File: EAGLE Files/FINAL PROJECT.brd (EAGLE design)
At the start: 100.3 x 49.5 mm, 15 parts, among them J1 BATTERY, U1 9_to_3.3_VREG

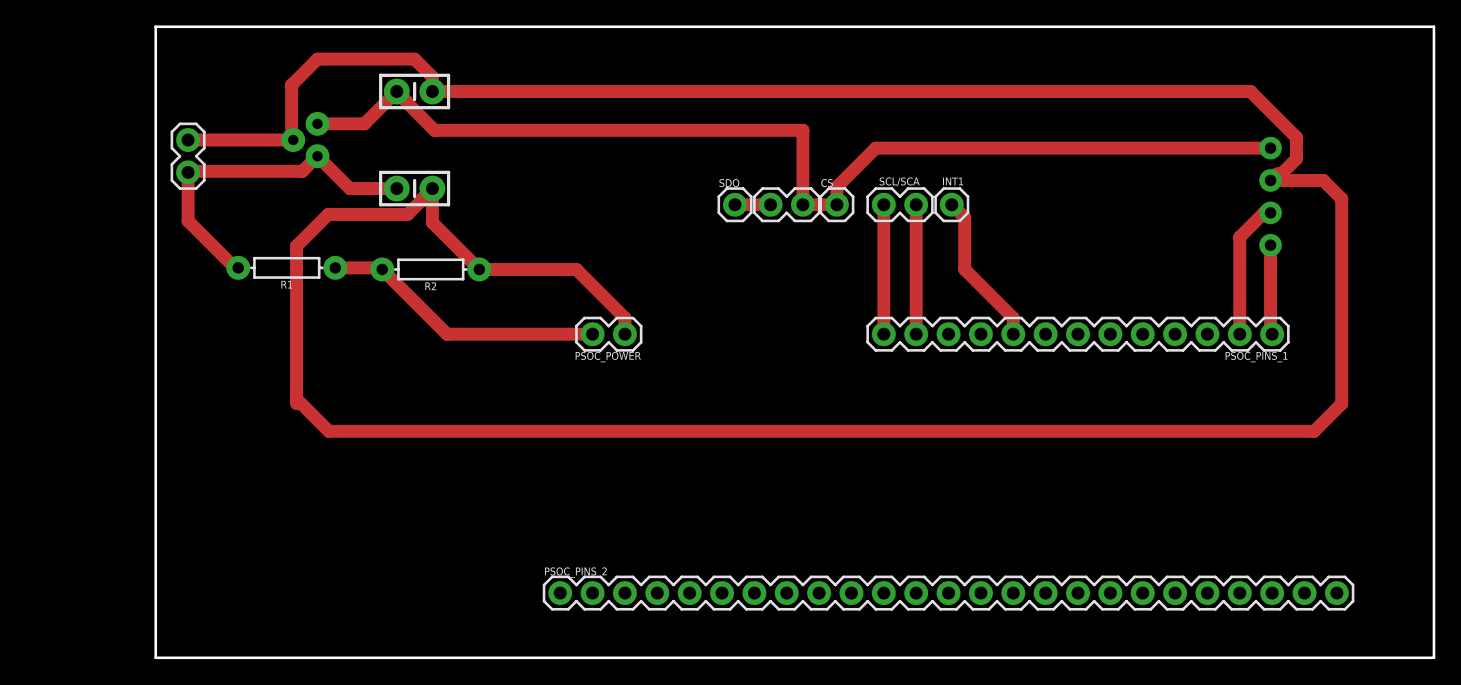
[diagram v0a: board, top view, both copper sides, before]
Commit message: FS and So code
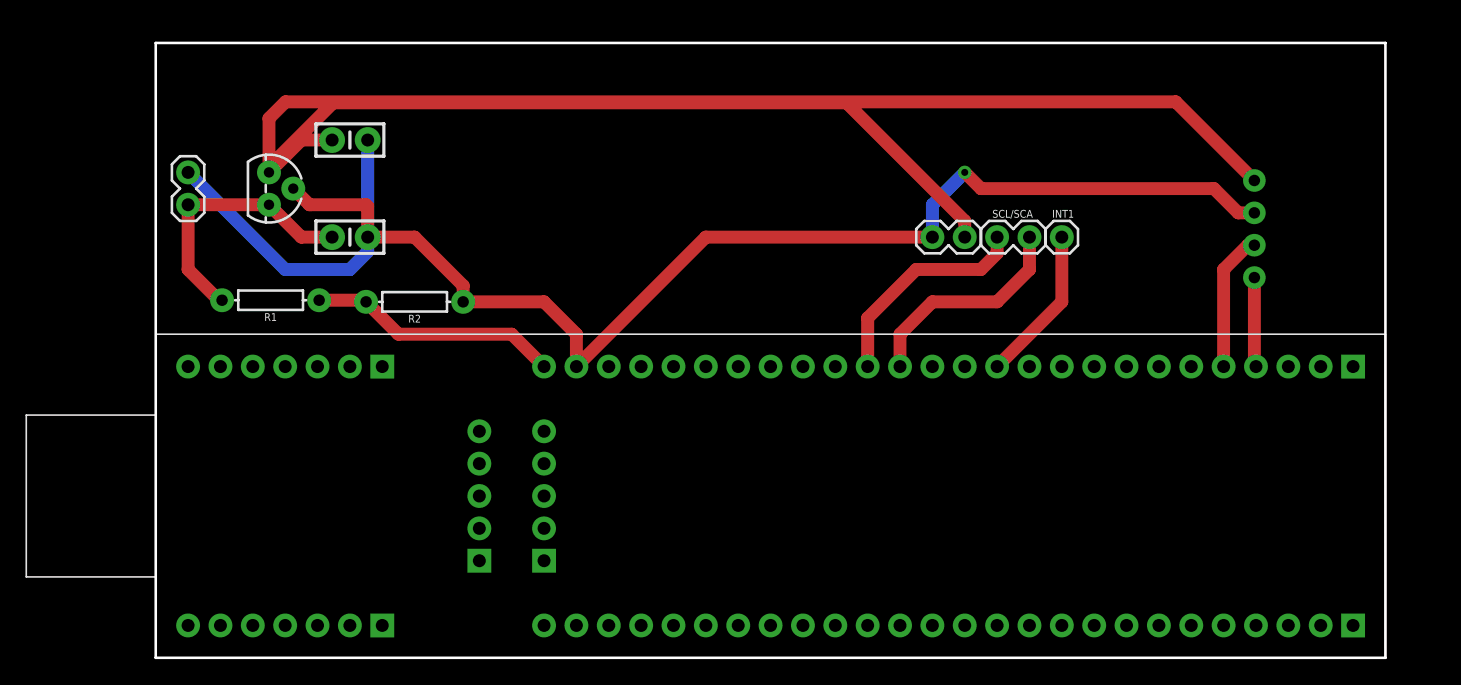
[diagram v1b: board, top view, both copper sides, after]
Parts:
- removed CS, SDO: (no value), SparkFun-Connectors:1X01
- removed PSOC_PINS_1: (no value), SparkFun-Connectors:1X13
- removed PSOC_PINS_2: (no value), SparkFun-Connectors:1X25
- removed PSOC_POWER: (no value), SparkFun-Connectors:1X02
- added U$1: CY8CKIT-059, CYKIT:CY8CKIT-059
- moved GND/VDD 13.0 mm to (61.0, 33.0)
- moved SCL/SCA 9.25 mm to (66.0, 33.0)
- moved INT1 9.00 mm to (71.1, 33.0)
- moved C3 6.35 mm to (15.2, 40.6)
- moved C4 6.35 mm to (15.2, 33.0)
- moved U1 5.39 mm to (8.89, 36.8), flipped to the top
- moved HC-05 2.84 mm to (102.7, 33.7)
- moved R1 2.84 mm to (9.02, 28.1)
- moved R2 2.84 mm to (20.3, 27.9)
- moved J1 2.54 mm to (2.54, 38.1)
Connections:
- net 5V: now also U$1.26; no longer PSOC_POWER.2
- net GND: now also U$1.25; no longer PSOC_POWER.1, SDO.1
- net INT1: now also U$1.12; no longer PSOC_PINS_1.9
- net RX: now also U$1.4; no longer PSOC_PINS_1.1
- net SCA: now also U$1.15; no longer PSOC_PINS_1.12
- net SCL: now also U$1.16; no longer PSOC_PINS_1.13
- net TX: now also U$1.5; no longer PSOC_PINS_1.2
- net VDD: no longer CS.1
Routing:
- net GND: track 256.4 -> 120.6 mm, vias 0 -> 1
- net VDD: track 85.7 -> 152.9 mm
- net SCL: track 10.2 -> 17.3 mm
- net SCA: track 10.2 -> 17.3 mm
- net VDD1: track 27.2 -> 21.1 mm
- net 5V: track 22.3 -> 19.8 mm
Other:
- board size 100.3 x 49.5 mm -> 96.5 x 48.3 mm

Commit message: update - EAGLE files
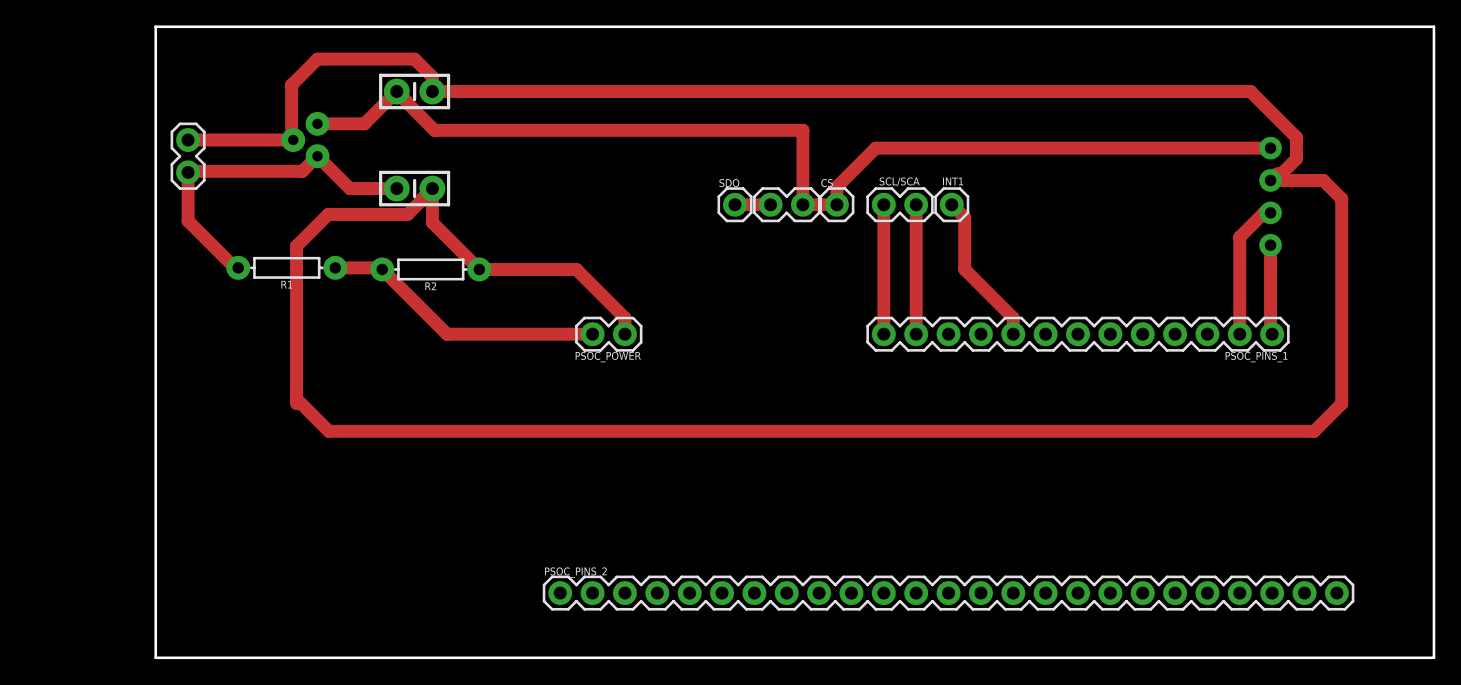
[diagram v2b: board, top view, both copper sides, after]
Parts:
- removed U$1: CY8CKIT-059, CYKIT:CY8CKIT-059
- added CS, SDO: (no value), SparkFun-Connectors:1X01
- added PSOC_PINS_1: (no value), SparkFun-Connectors:1X13
- added PSOC_PINS_2: (no value), SparkFun-Connectors:1X25
- added PSOC_POWER: (no value), SparkFun-Connectors:1X02
- moved GND/VDD 13.0 mm to (48.3, 35.6)
- moved SCL/SCA 9.25 mm to (57.1, 35.6)
- moved INT1 9.00 mm to (62.5, 35.6)
- moved C3 6.35 mm to (20.3, 44.5)
- moved C4 6.35 mm to (20.3, 36.8)
- moved U1 5.39 mm to (12.7, 40.6), flipped to the bottom
- moved HC-05 2.84 mm to (104.0, 36.2)
- moved R1 2.84 mm to (10.3, 30.6)
- moved R2 2.84 mm to (21.6, 30.5)
- moved J1 2.54 mm to (2.54, 40.6)
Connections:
- net 5V: now also PSOC_POWER.2; no longer U$1.26
- net GND: now also PSOC_POWER.1, SDO.1; no longer U$1.25
- net INT1: now also PSOC_PINS_1.9; no longer U$1.12
- net RX: now also PSOC_PINS_1.1; no longer U$1.4
- net SCA: now also PSOC_PINS_1.12; no longer U$1.15
- net SCL: now also PSOC_PINS_1.13; no longer U$1.16
- net TX: now also PSOC_PINS_1.2; no longer U$1.5
- net VDD: now also CS.1
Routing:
- net GND: track 120.6 -> 256.4 mm, vias 1 -> 0
- net VDD: track 152.9 -> 85.7 mm
- net SCL: track 17.3 -> 10.2 mm
- net SCA: track 17.3 -> 10.2 mm
- net VDD1: track 21.1 -> 27.2 mm
- net 5V: track 19.8 -> 22.3 mm
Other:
- board size 96.5 x 48.3 mm -> 100.3 x 49.5 mm
